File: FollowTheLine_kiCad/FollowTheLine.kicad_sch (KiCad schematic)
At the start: 11 parts, among them J1 Conn_01x02_Pin, J2 Conn_01x06_Pin, J3 Conn_01x05, J5 XT60-M, U1 ARDUINO_PRO_MINI, U3 L7805

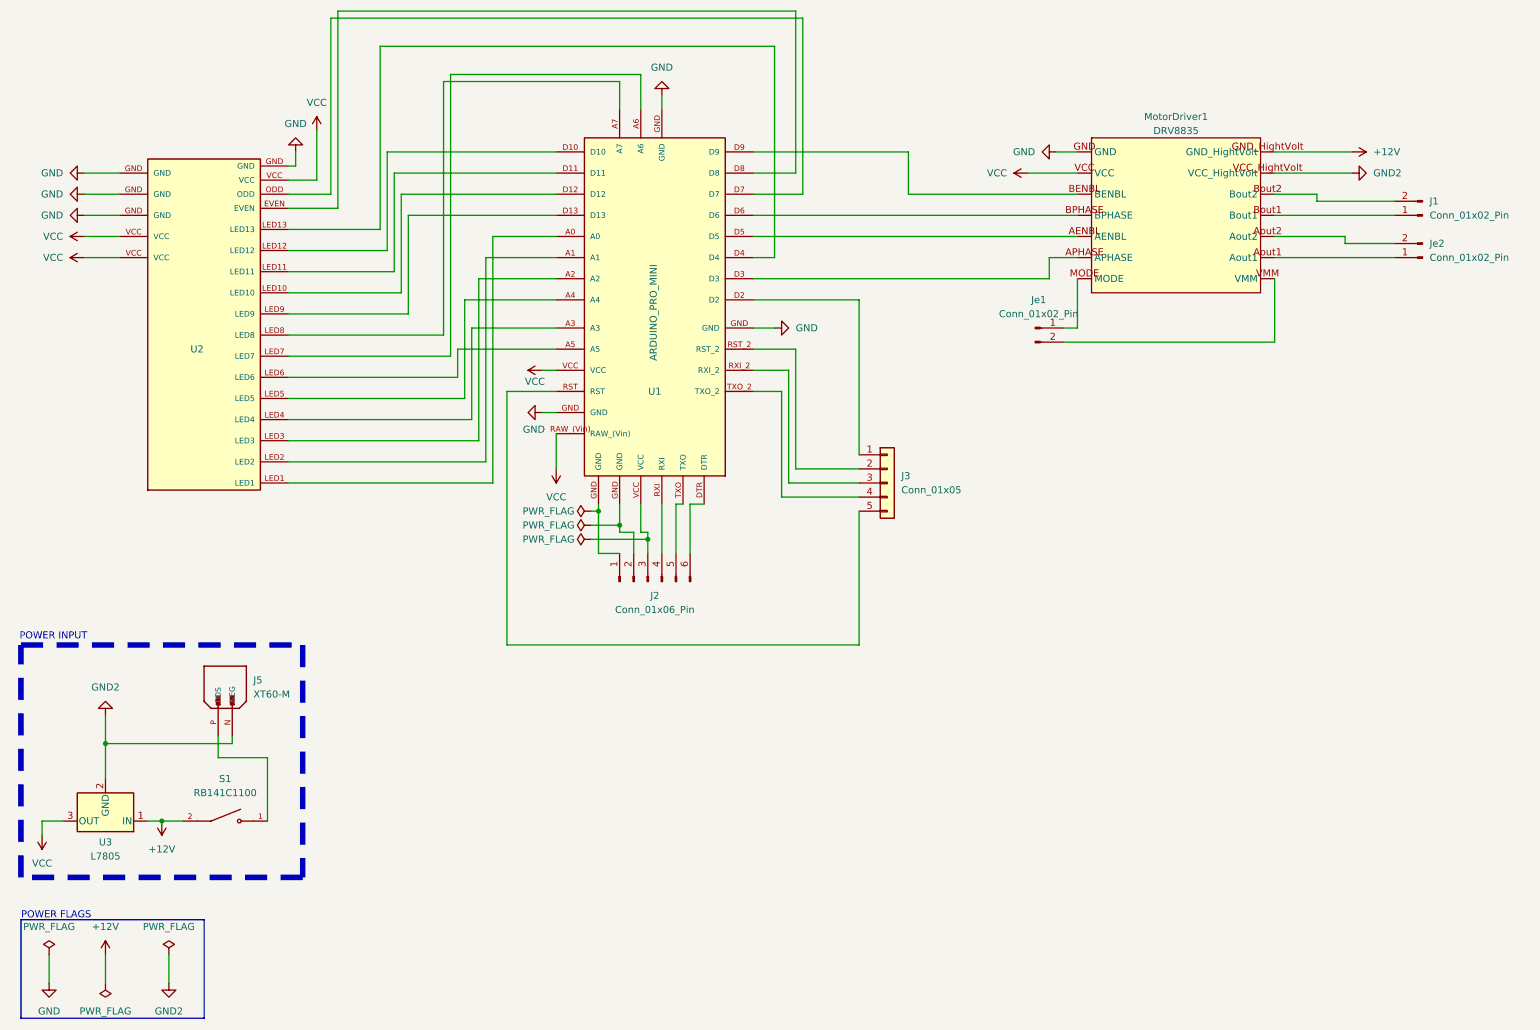
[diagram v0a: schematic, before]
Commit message: Follow the line. PCB version v2
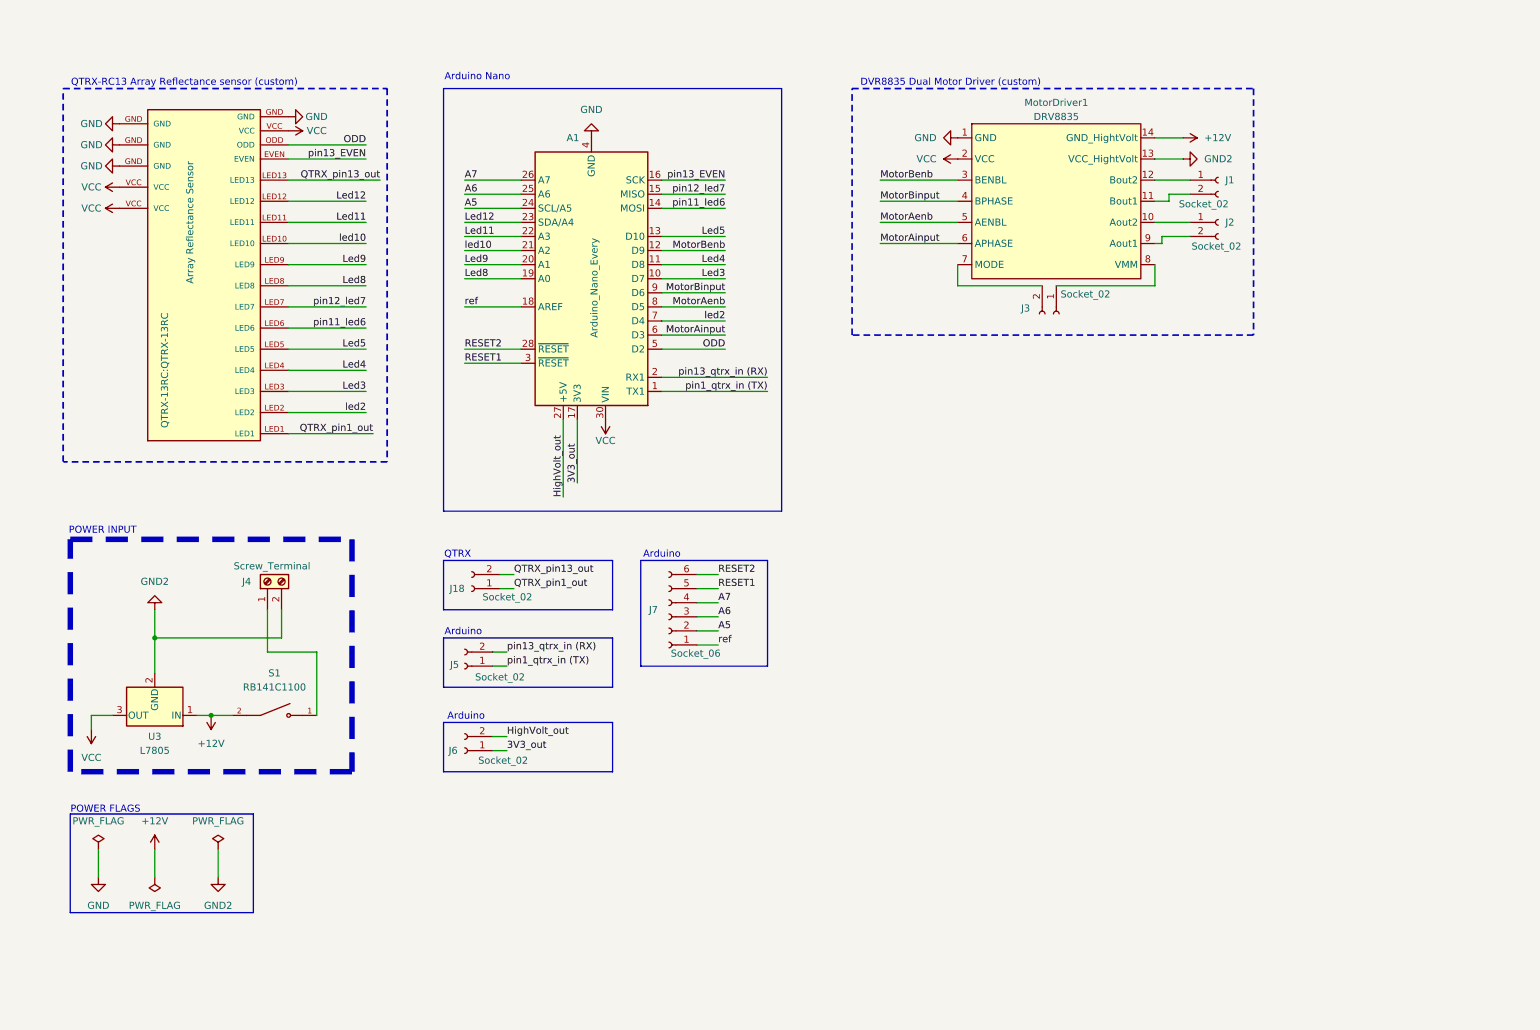
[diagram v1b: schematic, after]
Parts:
- removed J1, Je1, Je2: Conn_01x02_Pin, Connector_PinSocket_2.54mm:PinSocket_1x02_P2.54mm_Vertical, symbol Connector:Conn_01x02_Pin
- removed J2: Conn_01x06_Pin, Connector_PinSocket_2.54mm:PinSocket_1x06_P2.54mm_Vertical, symbol Connector:Conn_01x06_Pin
- removed J3: Conn_01x05, Connector_PinSocket_2.54mm:PinSocket_1x05_P2.54mm_Vertical, symbol Connector_Generic:Conn_01x05
- removed J5: XT60-M, XT60-M:AMASS_XT60-M, symbol XT60-M:XT60-M
- removed U1: ARDUINO_PRO_MINI, ARDUINO_PRO_MINI:MODULE_ARDUINO_PRO_MINI, symbol ARDUINO_PRO_MINI:ARDUINO_PRO_MINI
- added A1: Arduino_Nano_Every, Module:Arduino_Nano, symbol MCU_Module:Arduino_Nano_Every
- added J1, J18, J2, J3, J5, J6: Socket_02, Connector_PinSocket_2.54mm:PinSocket_1x02_P2.54mm_Vertical, symbol Connector:Conn_01x02_Socket
- added J4: Screw_Terminal, TerminalBlock_Phoenix:TerminalBlock_Phoenix_PTSM-0,5-2-2.5-V-THR_1x02_P2.50mm_Vertical, symbol Connector:Screw_Terminal_01x02
- added J7: Socket_06, Connector_PinSocket_2.54mm:PinSocket_1x06_P2.54mm_Vertical, symbol Connector:Conn_01x06_Socket
- MotorDriver1: footprint Library:DRV8835 -> Library:Driver_Motor
- U2: value ~ -> Array Reflectance Sensor; footprint QTR-8A:QTR-8A -> QTRX-13RC:QTRX-13RC
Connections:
- net +12V: now also MotorDriver1.14 (GND_HightVolt); no longer MotorDriver1.GND_HightVolt
- net GND: now also MotorDriver1.1 (GND), A1.29 (GND), A1.4 (GND); no longer MotorDriver1.GND
- net GND2: now also MotorDriver1.13 (VCC_HightVolt), J4.2 (Pin_2); no longer MotorDriver1.VCC_HightVolt
- net VCC: now also MotorDriver1.2 (VCC), A1.30 (VIN); no longer MotorDriver1.VCC
- net pin13_EVEN: now reaches U2.EVEN
- net pin13_EVEN: now also A1.16 (SCK)
- net QTRX_pin1_out: now reaches U2.LED1
- net QTRX_pin1_out: now also J18.1 (Pin_1)
- net led10: now reaches U2.LED10
- net led10: now also A1.21 (A2)
- net Led11: now reaches U2.LED11
- net Led11: now also A1.22 (A3)
- net Led12: now reaches U2.LED12
- net Led12: now also A1.23 (SDA/A4)
- net QTRX_pin13_out: now reaches U2.LED13
- net QTRX_pin13_out: now also J18.2 (Pin_2)
- net led2: now reaches U2.LED2
- net led2: now also A1.7 (D4)
- net Led3: now reaches U2.LED3
- net Led3: now also A1.10 (D7)
- net Led4: now reaches U2.LED4
- net Led4: now also A1.11 (D8)
- net Led5: now reaches U2.LED5
- net Led5: now also A1.13 (D10)
- net pin11_led6: now reaches U2.LED6
- net pin11_led6: now also A1.14 (MOSI)
- net pin12_led7: now reaches U2.LED7
- net pin12_led7: now also A1.15 (MISO)
- net Led8: now reaches U2.LED8
- net Led8: now also A1.19 (A0)
- net Led9: now reaches U2.LED9
- net Led9: now also A1.20 (A1)
- net ODD: now reaches U2.ODD
- net ODD: now also A1.5 (D2)
- net at S1.1: now also J4.1 (Pin_1)
- new net: J3.1 (Pin_1), MotorDriver1.8 (VMM)
- new net: J3.2 (Pin_2), MotorDriver1.7 (MODE)
- new net: J1.1 (Pin_1), MotorDriver1.12 (Bout2)
- new net: J1.2 (Pin_2), MotorDriver1.11 (Bout1)
- new net: J2.1 (Pin_1), MotorDriver1.10 (Aout2)
- new net: J2.2 (Pin_2), MotorDriver1.9 (Aout1)
- new net 3V3_out: A1.17 (3V3), J6.1 (Pin_1)
- new net A5: A1.24 (SCL/A5), J7.2 (Pin_2)
- new net A6: A1.25 (A6), J7.3 (Pin_3)
- new net A7: A1.26 (A7), J7.4 (Pin_4)
- new net HighVolt_out: A1.27 (+5V), J6.2 (Pin_2)
- new net MotorAenb: A1.8 (D5), MotorDriver1.5 (AENBL)
- new net MotorAinput: A1.6 (D3), MotorDriver1.6 (APHASE)
- new net MotorBenb: A1.12 (D9), MotorDriver1.3 (BENBL)
- new net MotorBinput: A1.9 (D6), MotorDriver1.4 (BPHASE)
- new net RESET1: A1.3 (~{RESET}), J7.5 (Pin_5)
- new net RESET2: A1.28 (~{RESET}), J7.6 (Pin_6)
- new net pin13_qtrx_in (RX): A1.2 (RX1), J5.2 (Pin_2)
- new net pin1_qtrx_in (TX): A1.1 (TX1), J5.1 (Pin_1)
- new net ref: A1.18 (AREF), J7.1 (Pin_1)
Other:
- note added: "Arduino"
- note added: "Arduino Nano"
- note added: "DVR8835 Dual Motor Driver (custom)"
- note added: "QTRX"
- note added: "QTRX-RC13 Array Reflectance sensor (custom)"
- moved on the sheet: MotorDriver1, S1, U3
